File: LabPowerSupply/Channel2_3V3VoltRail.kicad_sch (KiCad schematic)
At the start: 8 parts

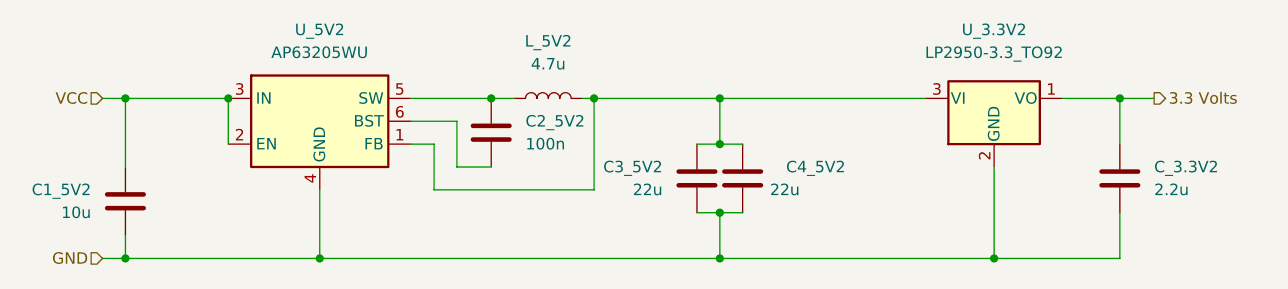
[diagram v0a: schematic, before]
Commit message: routing is weird
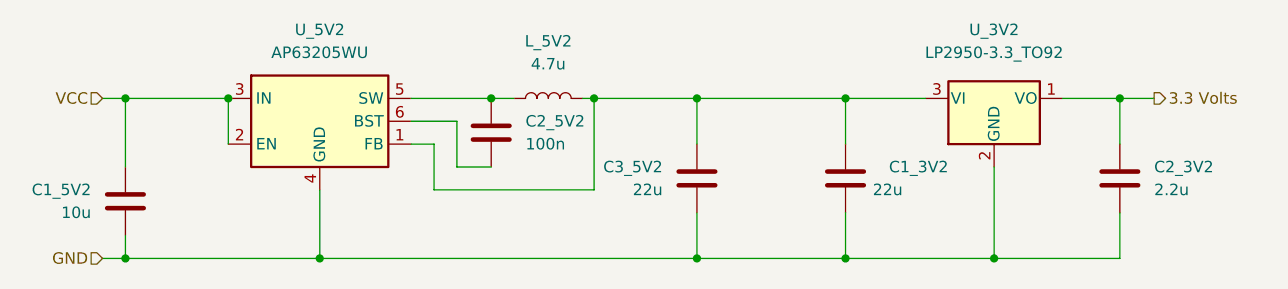
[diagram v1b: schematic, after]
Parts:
- renumbered C4_5V2 to C1_3V2, C_3.3V2 to C2_3V2, U_3.3V2 to U_3V2
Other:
- moved on the sheet: C1_3V2
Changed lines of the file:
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@@
   (junction (at 127 69.85) (diameter 0) (color 0 0 0 0)
   )
+  (junction (at 195.58 69.85) (diameter 0) (color 0 0 0 0)
+  )
   (junction (at 212.09 87.63) (diameter 0) (color 0 0 0 0)
   )
   (junction (at 115.57 69.85) (diameter 0) (color 0 0 0 0)
   )
-  (junction (at 181.61 82.55) (diameter 0) (color 0 0 0 0)
-  )
   (junction (at 167.64 69.85) (diameter 0) (color 0 0 0 0)
   )
+  (junction (at 195.58 87.63) (diameter 0) (color 0 0 0 0)
+  )
   (junction (at 226.06 69.85) (diameter 0) (color 0 0 0 0)
   )
   (junction (at 137.16 87.63) (diameter 0) (color 0 0 0 0)
   )
+  (junction (at 179.07 69.85) (diameter 0) (color 0 0 0 0)
+  )
   (junction (at 115.57 87.63) (diameter 0) (color 0 0 0 0)
   )
-  (junction (at 181.61 87.63) (diameter 0) (color 0 0 0 0)
-  )
-  (junction (at 181.61 69.85) (diameter 0) (color 0 0 0 0)
+  (junction (at 179.07 87.63) (diameter 0) (color 0 0 0 0)
   )
   (junction (at 156.21 69.85) (diameter 0) (color 0 0 0 0)
   )
-  (junction (at 181.61 74.93) (diameter 0) (color 0 0 0 0)
-  )
   (wire (pts (xy 167.64 69.85) (xy 167.64 80.01))
     (stroke (width 0) (type default) (color 0 0 0 0))
@@
     (stroke (width 0) (type default) (color 0 0 0 0))
   )
+  (wire (pts (xy 195.58 69.85) (xy 195.58 74.93))
+    (stroke (width 0) (type default) (color 0 0 0 0))
+  )
   (wire (pts (xy 226.06 82.55) (xy 226.06 87.63))
     (stroke (width 0) (type default) (color 0 0 0 0))
@@
     (stroke (width 0) (type default) (color 0 0 0 0))
   )
-  (wire (pts (xy 181.61 82.55) (xy 184.15 82.55))
-    (stroke (width 0) (type default) (color 0 0 0 0))
-  )
-  (wire (pts (xy 179.07 82.55) (xy 181.61 82.55))
+  (wire (pts (xy 195.58 69.85) (xy 204.47 69.85))
     (stroke (width 0) (type default) (color 0 0 0 0))
   )
@@
     (stroke (width 0) (type default) (color 0 0 0 0))
   )
+  (wire (pts (xy 195.58 87.63) (xy 212.09 87.63))
+    (stroke (width 0) (type default) (color 0 0 0 0))
+  )
   (wire (pts (xy 156.21 77.47) (xy 152.4 77.47))
     (stroke (width 0) (type default) (color 0 0 0 0))
   )
-  (wire (pts (xy 181.61 69.85) (xy 181.61 74.93))
-    (stroke (width 0) (type default) (color 0 0 0 0))
-  )
-  (wire (pts (xy 181.61 74.93) (xy 184.15 74.93))
-    (stroke (width 0) (type default) (color 0 0 0 0))
-  )
-  (wire (pts (xy 181.61 82.55) (xy 181.61 87.63))
+  (wire (pts (xy 179.07 69.85) (xy 179.07 74.93))
     (stroke (width 0) (type default) (color 0 0 0 0))
   )
@@
     (stroke (width 0) (type default) (color 0 0 0 0))
   )
+  (wire (pts (xy 179.07 69.85) (xy 195.58 69.85))
+    (stroke (width 0) (type default) (color 0 0 0 0))
+  )
   (wire (pts (xy 166.37 69.85) (xy 167.64 69.85))
     (stroke (width 0) (type default) (color 0 0 0 0))
   )
-  (wire (pts (xy 179.07 74.93) (xy 181.61 74.93))
-    (stroke (width 0) (type default) (color 0 0 0 0))
-  )
-  (wire (pts (xy 167.64 69.85) (xy 181.61 69.85))
+  (wire (pts (xy 167.64 69.85) (xy 179.07 69.85))
+    (stroke (width 0) (type default) (color 0 0 0 0))
+  )
+  (wire (pts (xy 179.07 82.55) (xy 179.07 87.63))
+    (stroke (width 0) (type default) (color 0 0 0 0))
+  )
+  (wire (pts (xy 195.58 82.55) (xy 195.58 87.63))
+    (stroke (width 0) (type default) (color 0 0 0 0))
+  )
+  (wire (pts (xy 179.07 87.63) (xy 195.58 87.63))
     (stroke (width 0) (type default) (color 0 0 0 0))
   )
@@
     (stroke (width 0) (type default) (color 0 0 0 0))
   )
-  (wire (pts (xy 181.61 69.85) (xy 204.47 69.85))
-    (stroke (width 0) (type default) (color 0 0 0 0))
-  )
   (wire (pts (xy 113.03 87.63) (xy 115.57 87.63))
     (stroke (width 0) (type default) (color 0 0 0 0))
   )
-  (wire (pts (xy 137.16 87.63) (xy 181.61 87.63))
-    (stroke (width 0) (type default) (color 0 0 0 0))
-  )
-  (wire (pts (xy 181.61 87.63) (xy 212.09 87.63))
+  (wire (pts (xy 137.16 87.63) (xy 179.07 87.63))
     (stroke (width 0) (type default) (color 0 0 0 0))
   )
@@
     (pin "6")
   )
-  (symbol (lib_id "Device:C") (at 184.15 78.74 0) (mirror x) (unit 1)
+  (symbol (lib_id "Device:C") (at 195.58 78.74 0) (mirror x) (unit 1)
     (in_bom yes) (on_board yes)
-    (property "Reference" "C4_5V2" (id 0) (at 195.58 77.47 0)
-      (effects (font (size 1.27 1.27)) (justify right))
-    )
-    (property "Value" "22u" (id 1) (at 190.5 80.01 0)
-      (effects (font (size 1.27 1.27)) (justify right))
-    )
-    (property "Footprint" "Capacitor_SMD:C_1210_3225Metric" (id 2) (at 185.1152 74.93 0)
-      (effects (font (size 1.27 1.27)) hide)
-    )
-    (property "Datasheet" "~" (id 3) (at 184.15 78.74 0)
+    (property "Reference" "C1_3V2" (id 0) (at 207.01 77.47 0)
+      (effects (font (size 1.27 1.27)) (justify right))
+    )
+    (property "Value" "22u" (id 1) (at 201.93 80.01 0)
+      (effects (font (size 1.27 1.27)) (justify right))
+    )
+    (property "Footprint" "Capacitor_SMD:C_1210_3225Metric" (id 2) (at 196.5452 74.93 0)
+      (effects (font (size 1.27 1.27)) hide)
+    )
+    (property "Datasheet" "~" (id 3) (at 195.58 78.74 0)
       (effects (font (size 1.27 1.27)) hide)
     )
@@
   (symbol (lib_id "Regulator_Linear:LP2950-3.3_TO92") (at 212.09 69.85 0) (unit 1)
     (in_bom yes) (on_board yes) (fields_autoplaced)
-    (property "Reference" "U_3.3V2" (id 0) (at 212.09 62.23 0))
+    (property "Reference" "U_3V2" (id 0) (at 212.09 62.23 0))
     (property "Value" "LP2950-3.3_TO92" (id 1) (at 212.09 64.77 0))
     (property "Footprint" "Package_TO_SOT_SMD:TO-252-3_TabPin4" (id 2) (at 212.09 64.135 0)
@@
   (symbol (lib_id "Device:C") (at 226.06 78.74 0) (unit 1)
     (in_bom yes) (on_board yes) (fields_autoplaced)
-    (property "Reference" "C_3.3V2" (id 0) (at 229.87 77.4699 0)
+    (property "Reference" "C2_3V2" (id 0) (at 229.87 77.4699 0)
       (effects (font (size 1.27 1.27)) (justify left))
     )
